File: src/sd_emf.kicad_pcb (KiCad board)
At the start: 2 copper layers, 60.7 x 43.3 mm, 10 parts, among them J1 Conn_01x01_Pin, Q1 2N3904, Q2 2N3904, Q3 2N3904, SW1 SW_Push

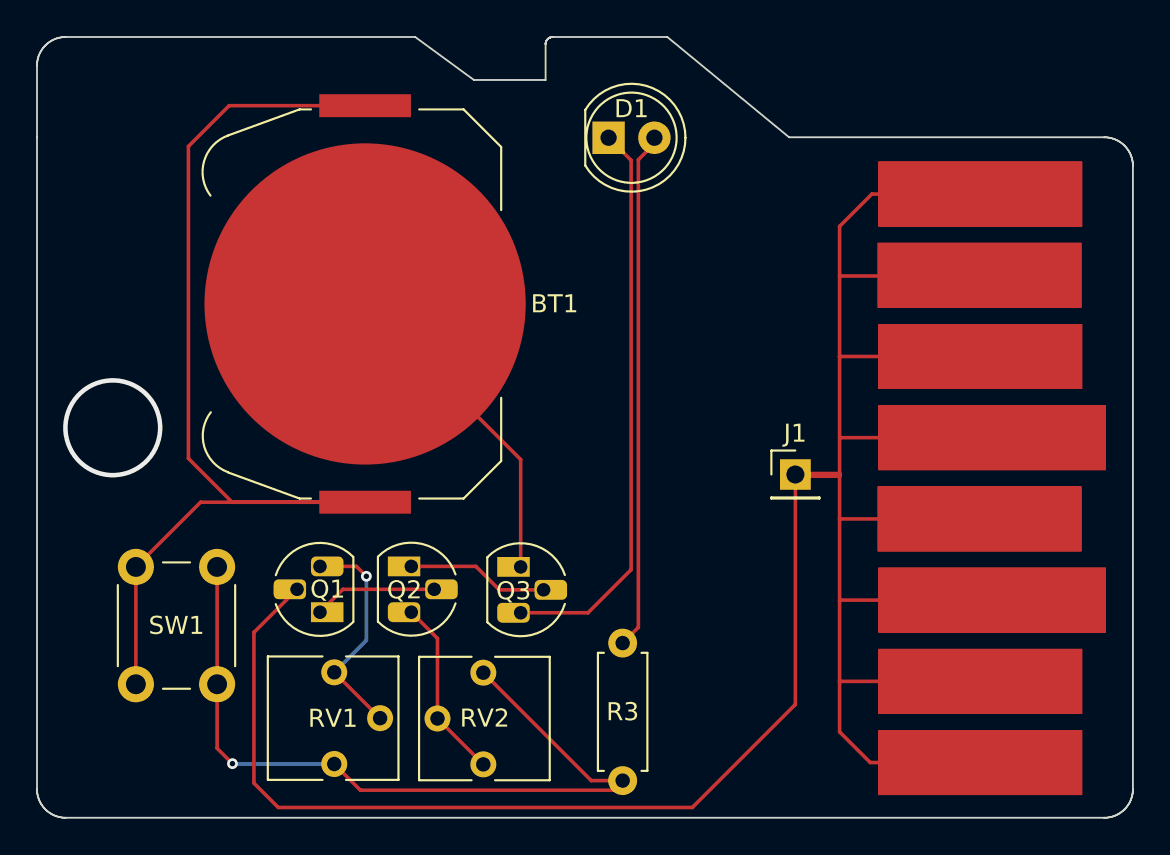
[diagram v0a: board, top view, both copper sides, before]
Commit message: feat: update pcb
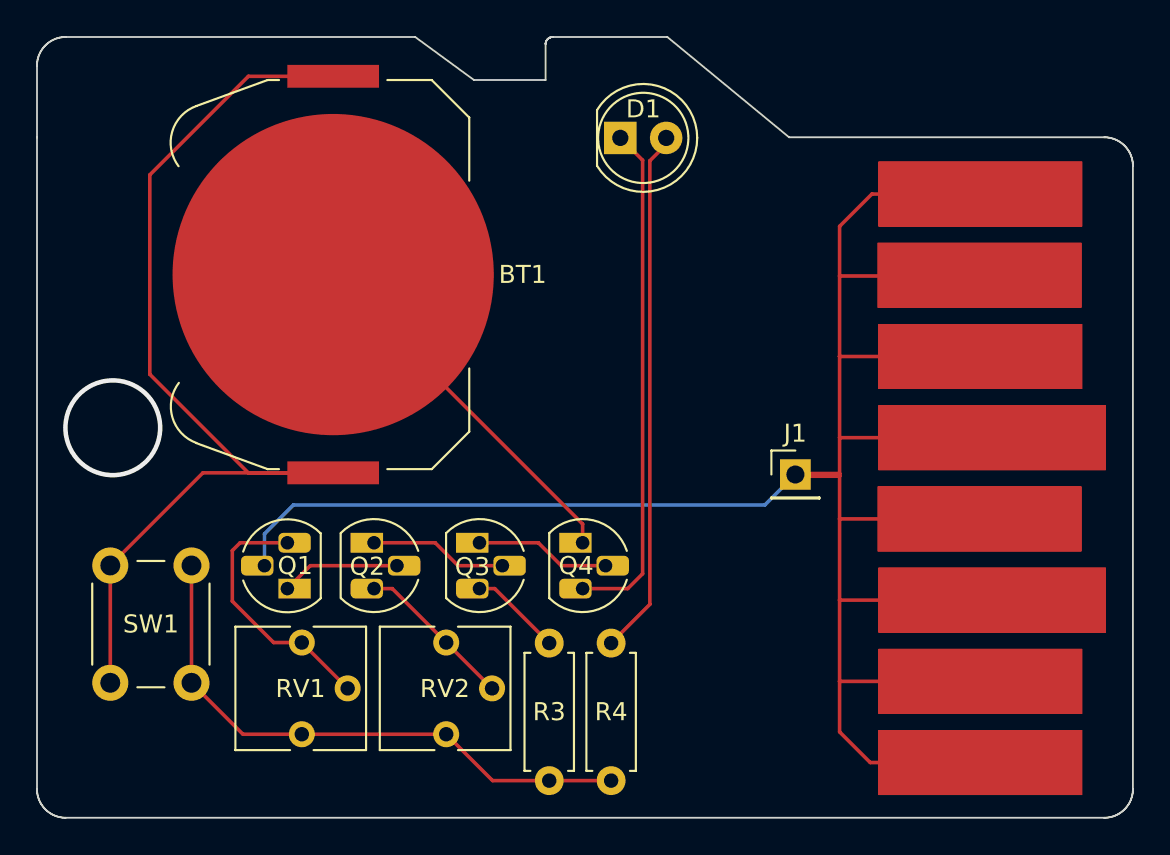
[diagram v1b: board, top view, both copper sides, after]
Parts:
- added Q4: 2N3904, Package_TO_SOT_THT:TO-92_HandSolder, F.Cu at (111.2, 72.1)
- added R4: 220, Resistor_THT:R_Axial_DIN0207_L6.3mm_D2.5mm_P7.62mm_Horizontal, F.Cu at (112.8, 85.3)
- R3: value 220 -> 4.7K
- moved R3 4.07 mm to (109.4, 85.3)
- moved RV2 3.98 mm to (103.7, 82.7), turned to 0 degrees
- moved Q3 2.65 mm to (105.5, 72.1)
- moved Q2 2.44 mm to (99.7, 72.1)
- moved RV1 2.44 mm to (95.7, 82.7)
- moved BT1 2.40 mm to (97.4, 57.3)
- moved Q1 2.23 mm to (94.9, 74.7)
- moved SW1 1.42 mm to (89.6, 73.4)
- moved D1 0.65 mm to (113.3, 49.7)
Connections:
- Q3 pad 1: Net-(BT1--) -> Net-(Q3-E)
- Q3 pad 3: Net-(D1-K) -> Net-(Q3-C)
- R3 pad 2: Net-(D1-A) -> Net-(Q3-C)
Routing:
- net Net-(J1-Pin_1): track 150.6 -> 125.8 mm
- net Net-(R3-Pad1): track 43.9 -> 32.2 mm, vias 1 -> 0
- net Net-(Q3-E): track 0.00 -> 7.51 mm
- net Net-(Q3-C): track 0.00 -> 5.12 mm
- net Net-(D1-K): track 31.6 -> 28.3 mm
- net Net-(BT1-+): track 59.5 -> 56.9 mm
- net Net-(BT1--): track 18.1 -> 20.6 mm
- net Net-(Q1-C): track 12.4 -> 14.4 mm, vias 1 -> 0
- net Net-(Q2-C): track 10.1 -> 8.83 mm
- net Net-(D1-A): track 28.7 -> 29.3 mm
